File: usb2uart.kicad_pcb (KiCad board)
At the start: 2 copper layers, 16 parts, among them P1 CONN_5, P2 CONN_2, P3 CONN_2, P4 CONN_2, P5 CONN_10

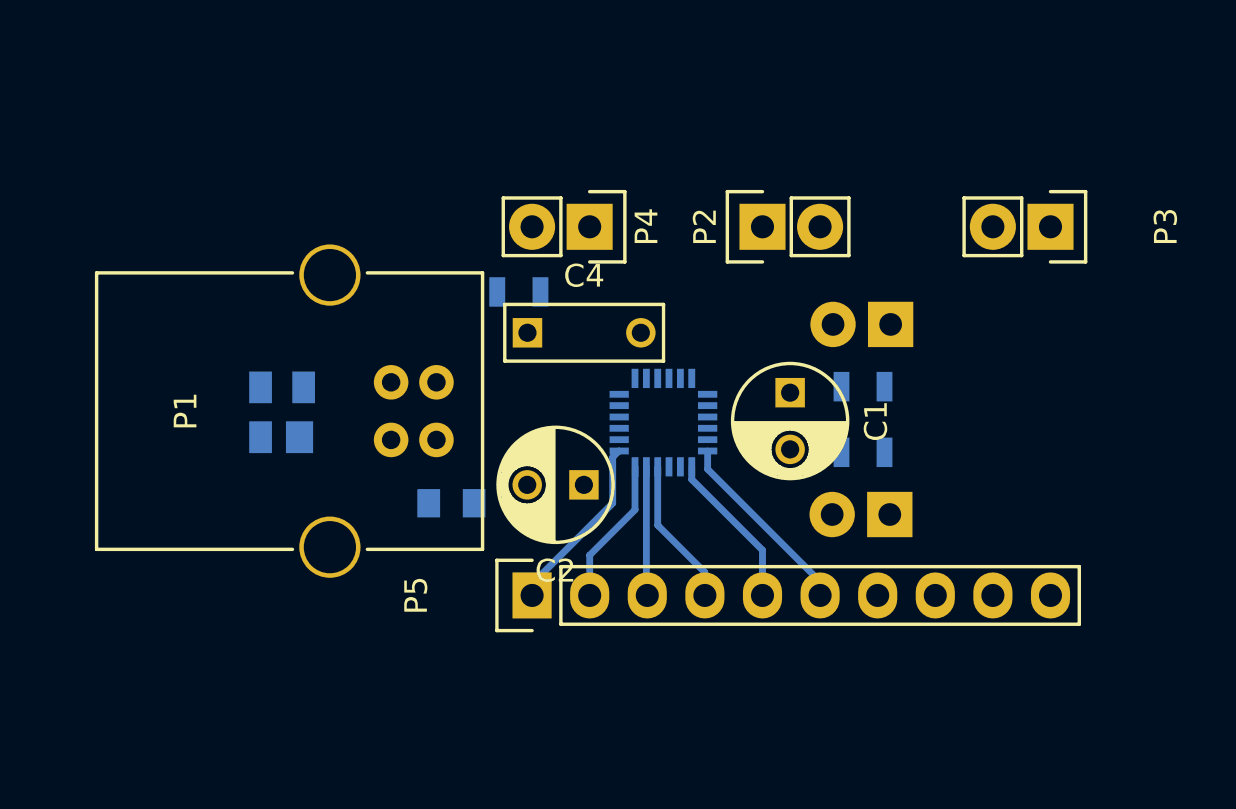
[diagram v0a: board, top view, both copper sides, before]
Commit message: Create board
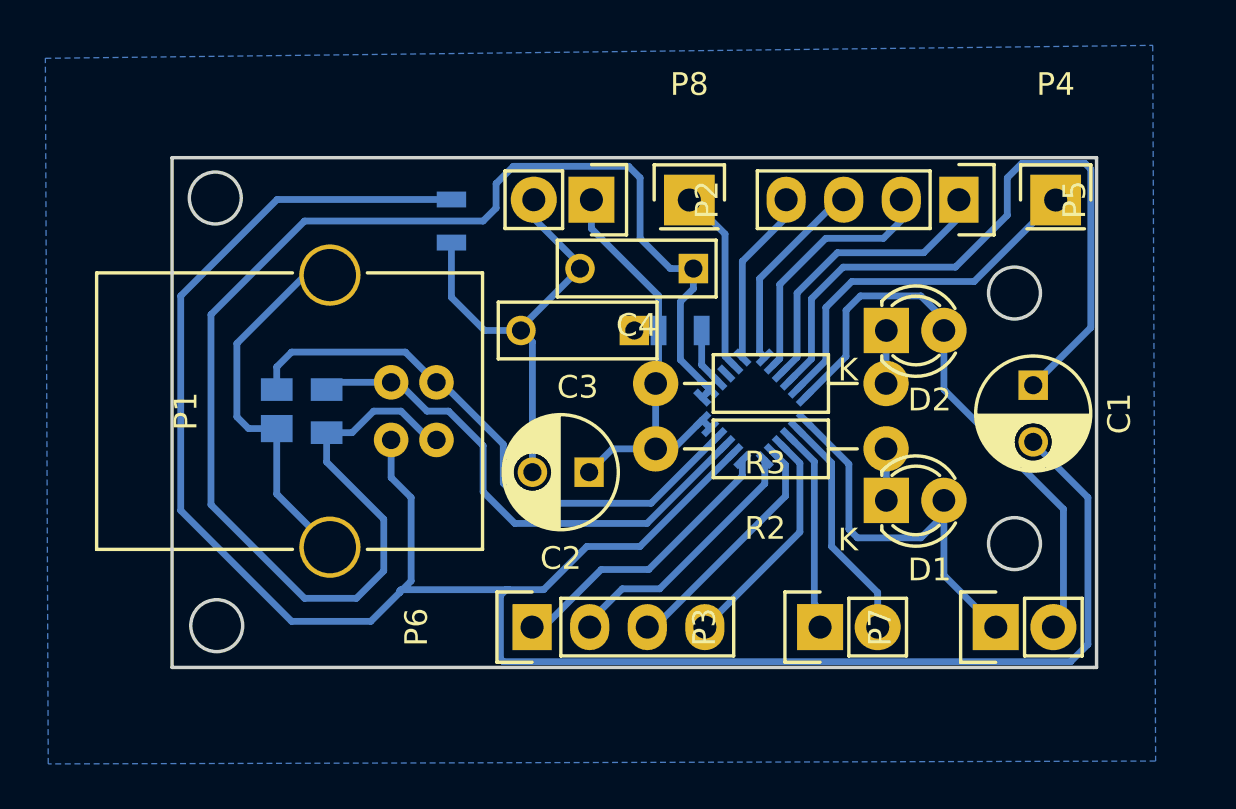
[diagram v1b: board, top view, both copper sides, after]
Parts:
- added P6: CONN_4, Pin_Headers:Pin_Header_Straight_1x04, F.Cu at (163.1, 117.5)
- added P7: CONN_2, Pin_Headers:Pin_Header_Straight_1x02, F.Cu at (183.5, 117.5)
- added P8: CONN_1, Pin_Headers:Pin_Header_Straight_1x01, F.Cu at (170.0, 98.6)
- added REF**: R_0805, Resistors_SMD:R_0805, B.Cu at (159.5, 99.6)
- C3: footprint Capacitors_SMD:C_0805 -> Capacitors_ThroughHole:C_Rect_L7_W2.5_P5; moved to F.Cu
- D1, D2: moved to F.Cu
- P4: value CONN_2 -> CONN_1; footprint Pin_Headers:Pin_Header_Straight_1x02 -> Pin_Headers:Pin_Header_Straight_1x01
- P5: value CONN_10 -> CONN_4; footprint Pin_Headers:Pin_Header_Straight_1x10 -> Pin_Headers:Pin_Header_Straight_1x04
- R2, R3: footprint Resistors_SMD:R_0805 -> Resistors_ThroughHole:Resistor_Horizontal_RM10mm; moved to F.Cu
- moved P5 25.7 mm to (181.9, 98.6), turned to 270 degrees
- moved P3 20.4 mm to (175.8, 117.5), turned to 90 degrees
- moved P4 13.0 mm to (186.2, 98.6), turned to 0 degrees
- moved C3 11.1 mm to (167.6, 104.4)
- moved C1 10.7 mm to (185.2, 106.8)
- moved C4 7.84 mm to (170.2, 101.7), turned to 180 degrees
- moved R1 7.31 mm to (169.6, 104.4)
- moved DD1 4.02 mm to (172.8, 107.8), turned to 45 degrees
- moved P2 1.20 mm to (165.7, 98.6)
- moved R2 1.03 mm to (178.7, 109.6), turned to 180 degrees
- moved R3 1.03 mm to (178.7, 106.7), turned to 180 degrees
- moved DA1 0.87 mm to (152.9, 108.0), turned to 90 degrees
- moved D1 0.64 mm to (178.7, 111.9), turned to 0 degrees
- moved C2 0.60 mm to (165.6, 110.6)
- moved D2 0.33 mm to (178.7, 104.4), turned to 0 degrees
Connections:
- DA1 pad 2: Net-(C4-Pad1) -> Net-(DA1-Pad2)
- DA1 pad 4: Net-(DA1-Pad4) -> Net-(C4-Pad1)
- DD1 pad 10: (no net) -> Net-(DD1-Pad10)
- DD1 pad 3: Net-(DA1-Pad4) -> Net-(DA1-Pad3)
- DD1 pad 4: Net-(DA1-Pad3) -> Net-(DA1-Pad2)
- P1 pad 2: Net-(DA1-Pad3) -> Net-(DA1-Pad2)
- P1 pad 3: Net-(DA1-Pad4) -> Net-(DA1-Pad3)
- P4 pad 1: Net-(DD1-Pad11) -> Net-(DD1-Pad17)
- P5 pad 1: Net-(DD1-Pad1) -> Net-(DD1-Pad15)
- P5 pad 2: Net-(DD1-Pad24) -> Net-(DD1-Pad14)
- P5 pad 3: Net-(DD1-Pad23) -> Net-(DD1-Pad13)
- P5 pad 4: Net-(DD1-Pad22) -> Net-(DD1-Pad12)
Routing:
- net Net-(C1-Pad2): track 0.00 -> 119.8 mm
- net Net-(C4-Pad1): track 0.00 -> 65.8 mm
- net Net-(C1-Pad1): track 0.00 -> 30.5 mm
- net Net-(DA1-Pad2): track 0.00 -> 25.7 mm
- net Net-(DA1-Pad3): track 0.00 -> 23.1 mm
- net Net-(C2-Pad1): track 0.00 -> 20.1 mm
- net Net-(DA1-Pad1): track 0.00 -> 16.8 mm
- net Net-(D2-Pad2): track 8.42 -> 25.1 mm
- net Net-(DD1-Pad17): track 0.00 -> 16.2 mm
- net Net-(DD1-Pad15): track 0.00 -> 13.1 mm
- net Net-(DD1-Pad14): track 0.00 -> 11.1 mm
- net Net-(D1-Pad2): track 6.96 -> 17.6 mm
- net Net-(DD1-Pad20): track 0.00 -> 10.3 mm
- net Net-(DD1-Pad21): track 0.00 -> 9.00 mm
- net Net-(DD1-Pad13): track 0.00 -> 8.72 mm
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- added copper zone on B.Cu, net Net-(C1-Pad2)
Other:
- board outline added: 40.8 x 22.5 mm
